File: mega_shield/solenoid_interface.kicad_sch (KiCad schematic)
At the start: 25 parts, among them J7 T4140012121-000, U10 NUP2202, U11 NUP2202, U12 NUP2202, U13 NUP2202, U9 NUP2202

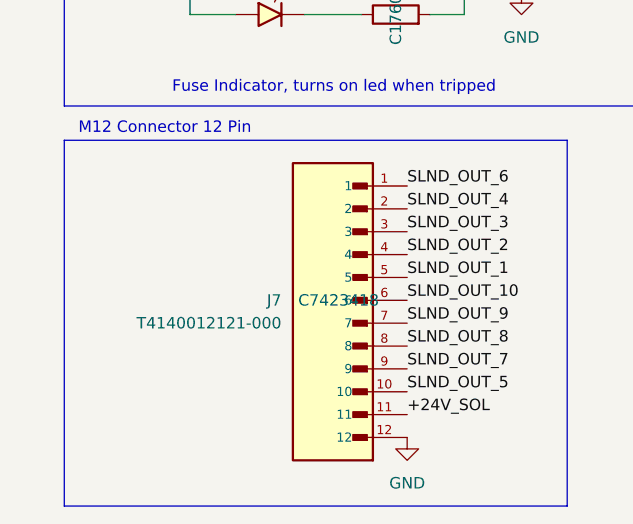
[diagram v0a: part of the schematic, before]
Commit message: mega_shield, Replaced Solenoid 12pin connector, re-arranged 0805 sized components, ran traces
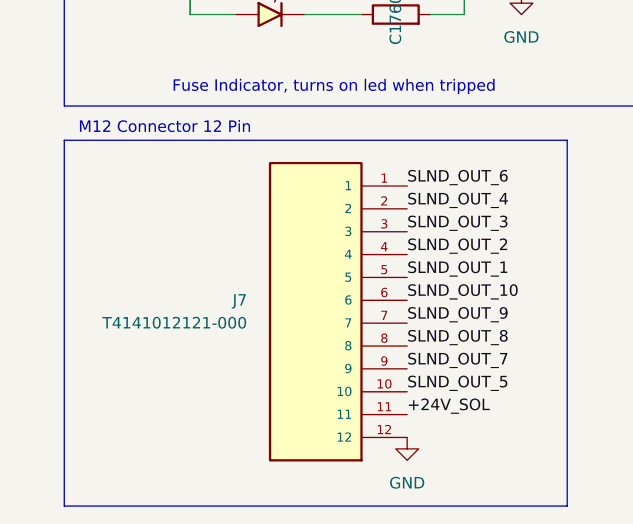
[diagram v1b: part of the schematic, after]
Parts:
- removed J7: T4140012121-000, footprints:TE_T4140012121-000, symbol M12P12:T4140012121-000
- added J7: T4141012121-000, footprints:TE_T4141012121-000, symbol mega_shield:T4141012121-000
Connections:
- net +24V_SOL: now also J7.11
- net GND: now also J7.12
- net SLND_OUT_1: now also J7.5
- net SLND_OUT_10: now also J7.6
- net SLND_OUT_2: now also J7.4
- net SLND_OUT_3: now also J7.3
- net SLND_OUT_4: now also J7.2
- net SLND_OUT_5: now also J7.10
- net SLND_OUT_6: now also J7.1
- net SLND_OUT_7: now also J7.9
- net SLND_OUT_8: now also J7.8
- net SLND_OUT_9: now also J7.7
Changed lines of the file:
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@@
-	)
-	(symbol
-		(lib_id "M12P12:T4140012121-000")
-		(at 55.88 144.78 0)
-		(mirror y)
-		(unit 1)
-		(exclude_from_sim no)
-		(in_bom yes)
-		(on_board yes)
-		(dnp no)
-		(property "Reference" "J7"
-			(at 49.53 144.7799 0)
-			(effects
-				(font
-					(size 1.27 1.27)
-				)
-				(justify left)
-			)
-		)
-		(property "Value" "T4140012121-000"
-			(at 49.53 147.3199 0)
-			(effects
-				(font
-					(size 1.27 1.27)
-				)
-				(justify left)
-			)
-		)
-		(property "Footprint" "footprints:TE_T4140012121-000"
-			(at 55.88 144.78 0)
-			(effects
-				(font
-					(size 1.27 1.27)
-				)
-				(justify bottom)
-				(hide yes)
-			)
-		)
-		(property "Datasheet" ""
-			(at 55.88 144.78 0)
-			(effects
-				(font
-					(size 1.27 1.27)
-				)
-				(hide yes)
-			)
-		)
-		(property "Description" ""
-			(at 55.88 144.78 0)
-			(effects
-				(font
-					(size 1.27 1.27)
-				)
-				(hide yes)
-			)
-		)
-		(property "PARTREV" "B"
-			(at 55.88 144.78 0)
-			(effects
-				(font
-					(size 1.27 1.27)
-				)
-				(justify bottom)
-				(hide yes)
-			)
-		)
-		(property "STANDARD" "Manufacturer Recommendations"
-			(at 55.88 144.78 0)
-			(effects
-				(font
-					(size 1.27 1.27)
-				)
-				(justify bottom)
-				(hide yes)
-			)
-		)
-		(property "MAXIMUM_PACKAGE_HEIGHT" "23mm"
-			(at 55.88 144.78 0)
-			(effects
-				(font
-					(size 1.27 1.27)
-				)
-				(justify bottom)
-				(hide yes)
-			)
-		)
-		(property "MANUFACTURER" "TE Connectivity"
-			(at 55.88 144.78 0)
-			(effects
-				(font
-					(size 1.27 1.27)
-				)
-				(justify bottom)
-				(hide yes)
-			)
-		)
-		(property "jlcpcb" "C7423418"
-			(at 55.88 144.78 0)
-			(effects
-				(font
-					(size 1.27 1.27)
-				)
-			)
-		)
-		(property "Sim.Device" ""
-			(at 55.88 144.78 0)
-			(effects
-				(font
-					(size 1.27 1.27)
-				)
-				(hide yes)
-			)
-		)
-		(property "Sim.Pins" ""
-			(at 55.88 144.78 0)
-			(effects
-				(font
-					(size 1.27 1.27)
-				)
-				(hide yes)
-			)
-		)
-		(property "Sim.Type" ""
-			(at 55.88 144.78 0)
-			(effects
-				(font
-					(size 1.27 1.27)
-				)
-				(hide yes)
-			)
-		)
-		(pin "9"
-		)
-		(pin "8"
-		)
-		(pin "12"
-		)
-		(pin "4"
-		)
-		(pin "5"
-		)
-		(pin "6"
-		)
-		(pin "7"
-		)
-		(pin "3"
-		)
-		(pin "11"
-		)
-		(pin "10"
-		)
-		(pin "2"
-		)
-		(pin "1"
-		)
-		(instances
-			(project ""
-				(path "/554fcf27-dc63-4666-abbc-7481d15942c4/2699417b-945f-4287-8f74-1d8b0d60679f"
-					(reference "J7")
-					(unit 1)
-				)
-			)
-		)
 	)
 	(symbol
@@
 					(unit 1)
 				)
+			)
+		)
+	)
+	(symbol
+		(lib_id "mega_shield:T4141012121-000")
+		(at 53.34 144.78 0)
+		(mirror y)
+		(unit 1)
+		(exclude_from_sim no)
+		(in_bom yes)
+		(on_board yes)
+		(dnp no)
+		(property "Reference" "J7"
+			(at 45.72 144.7799 0)
+			(effects
+				(font
+					(size 1.27 1.27)
+				)
+				(justify left)
+			)
+		)
+		(property "Value" "T4141012121-000"
+			(at 45.72 147.3199 0)
+			(effects
+				(font
+					(size 1.27 1.27)
+				)
+				(justify left)
+			)
+		)
+		(property "Footprint" "footprints:TE_T4141012121-000"
+			(at 53.34 144.78 0)
+			(effects
+				(font
+					(size 1.27 1.27)
+				)
+				(justify bottom)
+				(hide yes)
+			)
+		)
+		(property "Datasheet" ""
+			(at 53.34 144.78 0)
+			(effects
+				(font
+					(size 1.27 1.27)
+				)
+				(hide yes)
+			)
+		)
+		(property "Description" ""
+			(at 53.34 144.78 0)
+			(effects
+				(font
+					(size 1.27 1.27)
+				)
+				(hide yes)
+			)
+		)
+		(property "PARTREV" "B"
+			(at 53.34 144.78 0)
+			(effects
+				(font
+					(size 1.27 1.27)
+				)
+				(justify bottom)
+				(hide yes)
+			)
+		)
+		(property "MANUFACTURER" "TE Connectivity"
+			(at 53.34 144.78 0)
+			(effects
+				(font
+					(size 1.27 1.27)
+				)
+				(justify bottom)
+				(hide yes)
+			)
+		)
+		(property "MAXIMUM_PACKAGE_HEIGHT" "20.0mm"
+			(at 53.34 144.78 0)
+			(effects
+				(font
+					(size 1.27 1.27)
+				)
+				(justify bottom)
+				(hide yes)
+			)
+		)
+		(property "STANDARD" "Manufacturer recommendations"
+			(at 53.34 144.78 0)
+			(effects
+				(font
+					(size 1.27 1.27)
+				)
+				(justify bottom)
+				(hide yes)
+			)
+		)
+		(pin "11"
+		)
+		(pin "9"
+		)
+		(pin "1"
+		)
+		(pin "2"
+		)
+		(pin "3"
+		)
+		(pin "4"
+		)
+		(pin "5"
+		)
+		(pin "10"
+		)
+		(pin "12"
+		)
+		(pin "8"
+		)
+		(pin "7"
+		)
+		(pin "6"
+		)
+		(instances
+			(project ""
+				(path "/554fcf27-dc63-4666-abbc-7481d15942c4/2699417b-945f-4287-8f74-1d8b0d60679f"
+					(reference "J7")
+					(unit 1)
+				)
